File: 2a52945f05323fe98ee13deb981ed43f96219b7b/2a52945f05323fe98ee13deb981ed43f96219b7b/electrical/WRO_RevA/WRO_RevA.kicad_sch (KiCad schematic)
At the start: 29 parts, among them J1 MPU6050, J1 VCC, J2 Conn_01x05_Pin, SW1 EXEC_PRGM, U1 ESP32-DEVKIT-V1, U2 ROB-14450

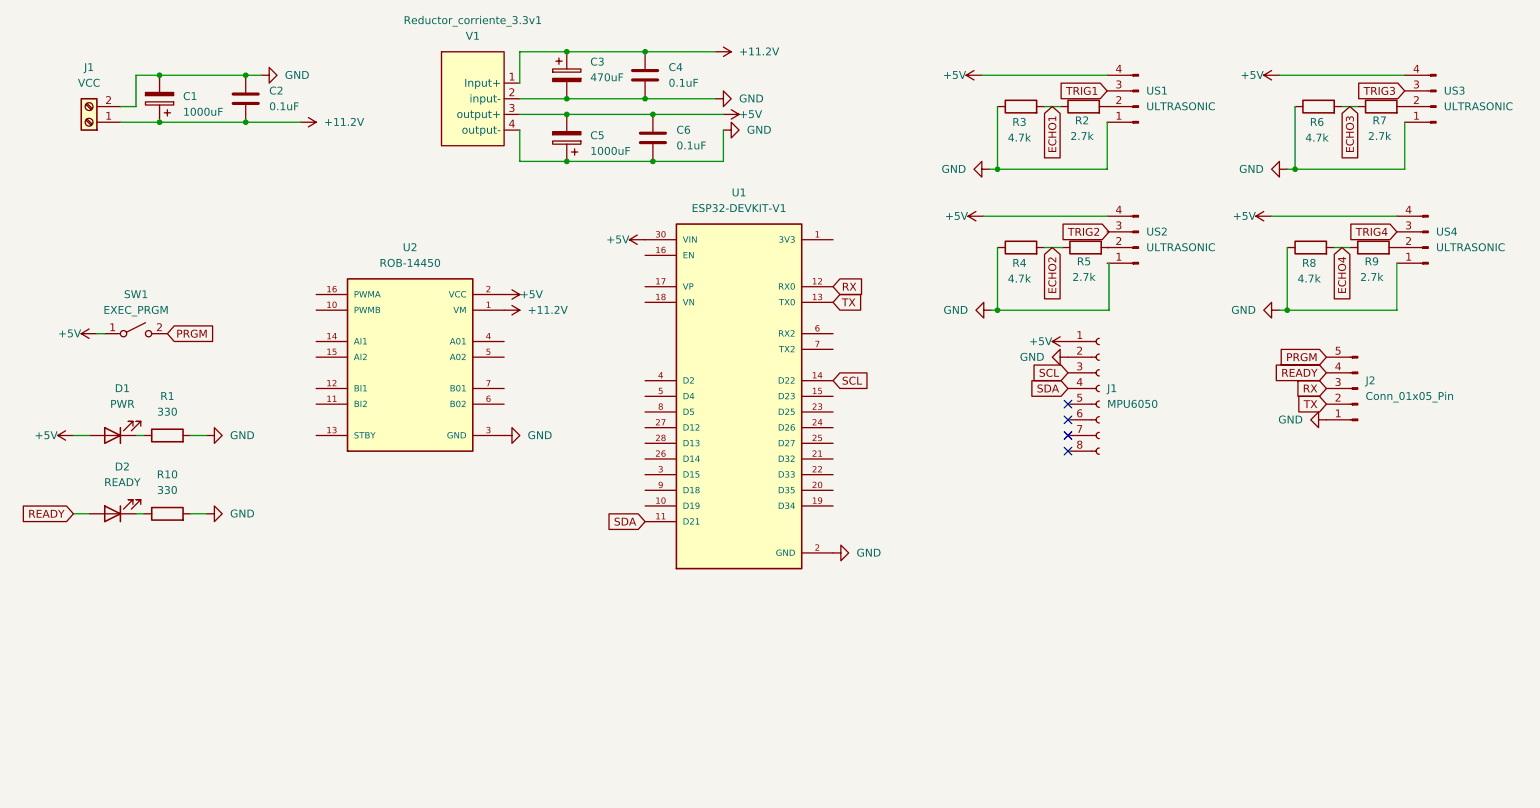
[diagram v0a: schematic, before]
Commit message: schematic done
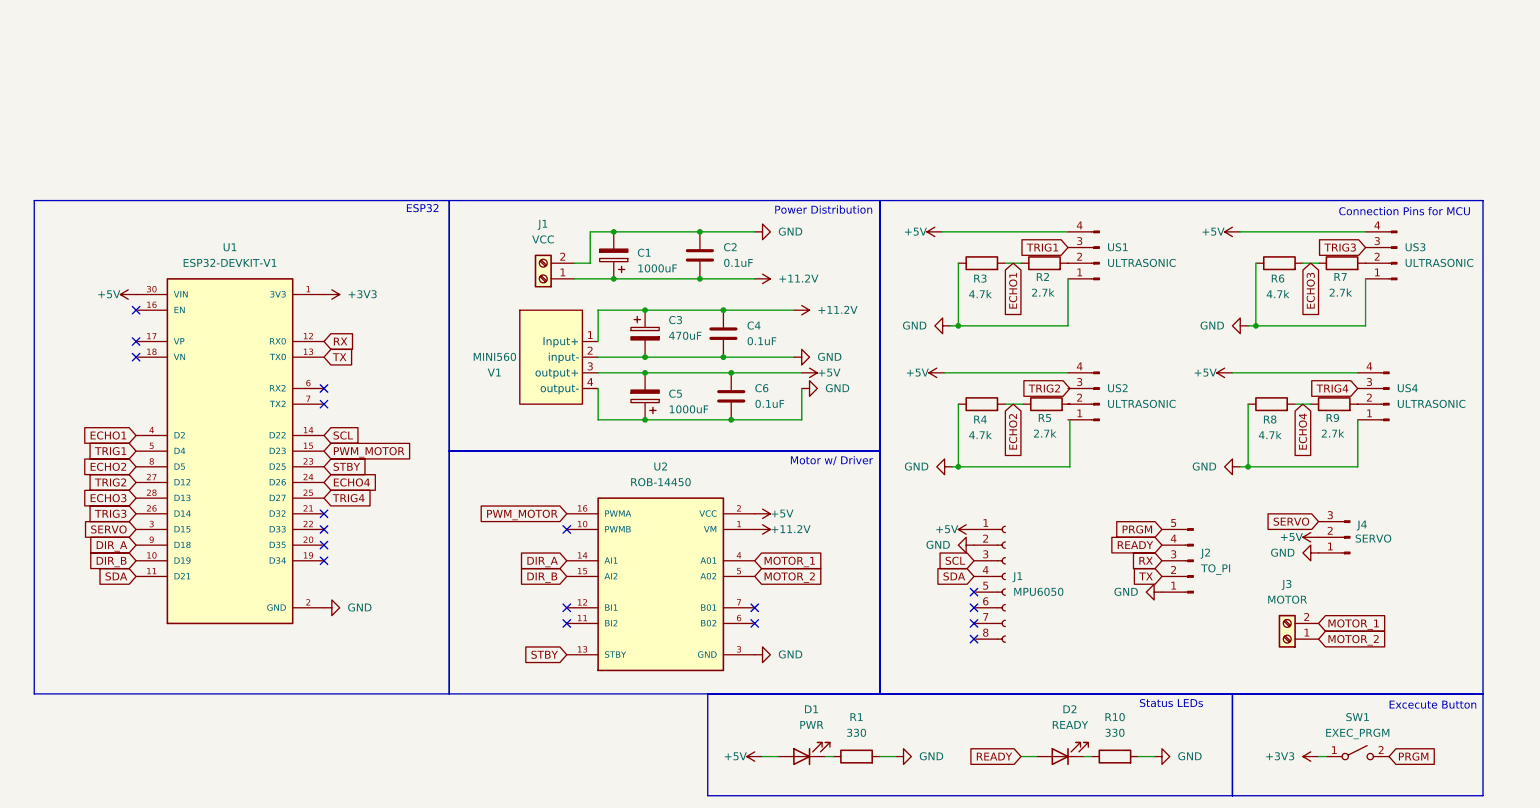
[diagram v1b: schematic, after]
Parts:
- added J3: MOTOR, TerminalBlock_Phoenix:TerminalBlock_Phoenix_PT-1,5-2-5.0-H_1x02_P5.00mm_Horizontal, symbol Connector:Screw_Terminal_01x02
- added J4: SERVO, Connector_PinSocket_2.54mm:PinSocket_1x03_P2.54mm_Vertical, symbol Connector:Conn_01x03_Pin
- J2: value Conn_01x05_Pin -> TO_PI
- renumbered Reductor_corriente_3.3v1 to MINI560
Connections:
- net +5V: now also J4.2 (Pin_2); no longer SW1.1 (A)
- net ECHO1: now also U1.4 (D2)
- net ECHO2: now also U1.8 (D5)
- net ECHO3: now also U1.28 (D13)
- net ECHO4: now also U1.24 (D26)
- net GND: now also J4.1 (Pin_1)
- net TRIG1: now also U1.5 (D4)
- net TRIG2: now also U1.27 (D12)
- net TRIG3: now also U1.26 (D14)
- net TRIG4: now also U1.25 (D27)
- net STBY: now reaches U2.13 (STBY)
- net STBY: now also U1.23 (D25)
- net DIR_A: now reaches U2.14 (AI1)
- net DIR_A: now also U1.9 (D18)
- net DIR_B: now reaches U2.15 (AI2)
- net DIR_B: now also U1.10 (D19)
- net PWM_MOTOR: now reaches U2.16 (PWMA)
- net PWM_MOTOR: now also U1.15 (D23)
- net MOTOR_1: now reaches U2.4 (A01)
- net MOTOR_1: now also J3.2 (Pin_2)
- net MOTOR_2: now reaches U2.5 (A02)
- net MOTOR_2: now also J3.1 (Pin_1)
- net +3V3: now reaches U1.1 (3V3)
- net +3V3: now also SW1.1 (A)
- net SERVO: now reaches U1.3 (D15)
- net SERVO: now also J4.3 (Pin_3)
- no-connect marks 4 -> 18
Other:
- note added: "Connection Pins for MCU"
- note added: "ESP32"
- note added: "Excecute Button"
- note added: "Motor w/ Driver"
- note added: "Power Distribution"
- note added: "Status LEDs"
- moved on the sheet: C1, C2, C3, C4, C5, C6, D1, D2, J1, J2, MINI560, R1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
